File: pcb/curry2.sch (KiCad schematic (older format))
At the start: 30 parts

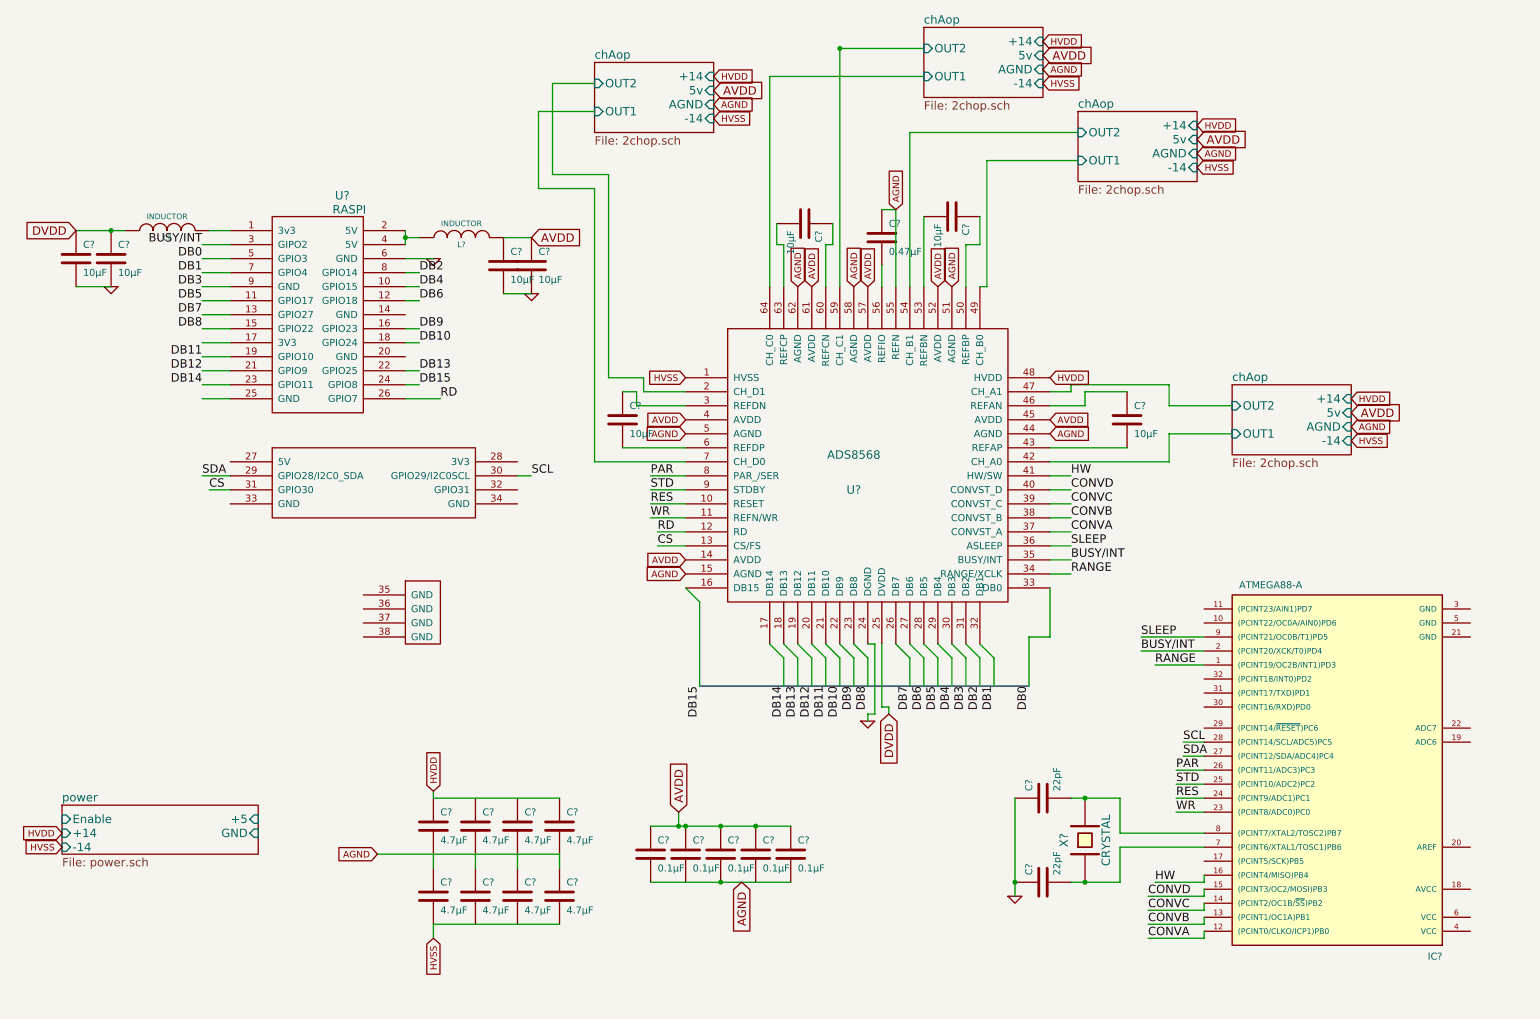
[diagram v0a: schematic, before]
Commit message: almost done rtc placed
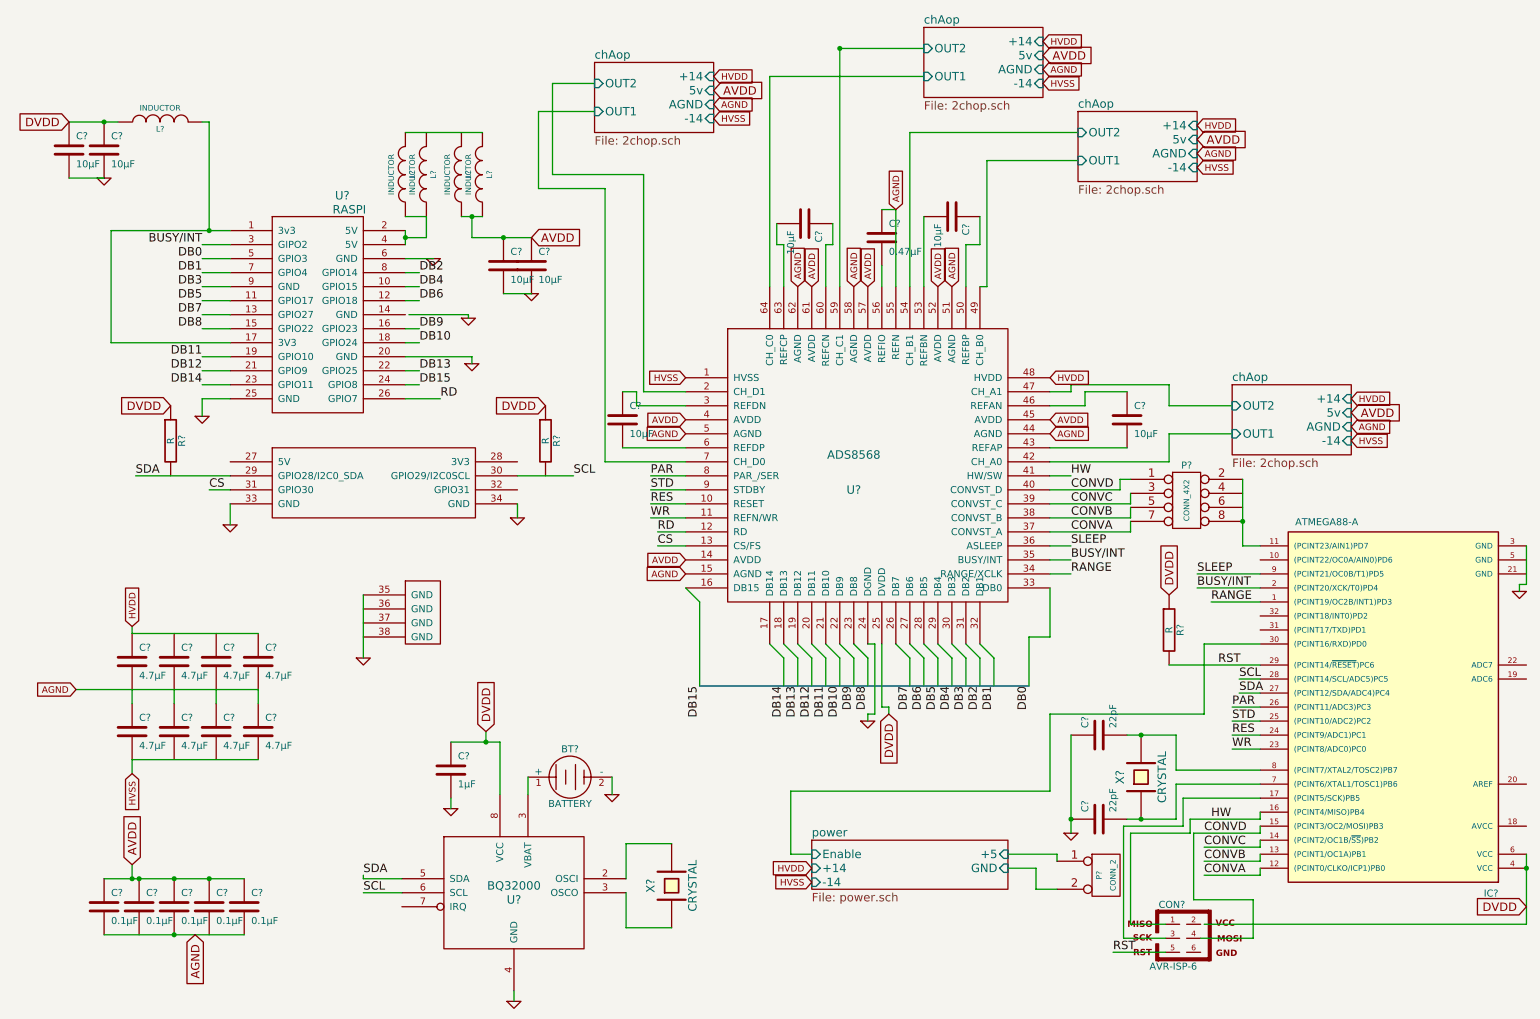
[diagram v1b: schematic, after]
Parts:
- added BT?: BATTERY, symbol BATTERY
- added C?: 1µF, symbol C
- added CON?: AVR-ISP-6, AVR-ISP-6, symbol AVR-ISP-6
- added L? (x3): INDUCTOR, symbol INDUCTOR
- added P?: CONN_2, symbol CONN_2
- added P?: CONN_4X2, symbol CONN_4X2
- added R? (x3): R, symbol R
- added U?: BQ32000, symbol BQ32000
- added X?: CRYSTAL, symbol CRYSTAL
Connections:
- net chAop/OUT1 is gone; now on net chAop/OUT1: U?.7 (CH_D0)
- net chAop/OUT2 is gone; now on net chAop/OUT2: U?.59 (CH_C1)
- net AVDD: now also L?.1, L?.1; no longer L?.2
- net CONVA: now also P?.7
- net CONVB: now also P?.5
- net CONVC: now also P?.3
- net CONVD: now also CON?.4, P?.1
- net DVDD: now also IC?.4 (VCC), IC?.6 (VCC), C?.1, R?.1, R?.1, R?.1, U?.8 (VCC)
- net GND: now also IC?.3 (GND), U?.20 (GND), U?.25 (GND), U?.33 (GND), U?.34 (GND), U?.35 (GND), BT?.2 (-), C?.2, U?.4 (GND)
- net HW: now also CON?.1
- net SCL: now also U?.6 (SCL)
- net SDA: now also U?.5 (SDA)
- net chAop/OUT1: no longer U?.42 (CH_A0)
- net chAop/OUT2: no longer U?.2 (CH_D1)
- net power/+5: now also P?.1 (P1)
- net power/Enable: now also IC?.30 ((PCINT16/RXD)PD0)
- net power/GND: now also P?.2 (PM)
- net at L?.2, U?.1 (3v3): now also U?.17 (3V3)
- net at L?.1, U?.2 (5V), U?.4 (5V): now also L?.1
- net at IC?.11 ((PCINT23/AIN1)PD7): now also P?.2, P?.8
- net at IC?.17 ((PCINT5/SCK)PB5): now also CON?.3
- net RST: now reaches IC?.29 ((PCINT14/~RESET~)PC6)
- net RST: now also CON?.5, R?.2
- new net: L?.2, L?.2
- new net: U?.2 (OSCI), X?.2
- new net: BT?.1 (+), U?.3 (VBAT)
- new net: U?.3 (VBAT), X?.1
- new net chAop/OUT1: U?.42 (CH_A0)
- new net chAop/OUT2: U?.2 (CH_D1)
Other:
- moved on the sheet: C?, IC?, L?, X?
